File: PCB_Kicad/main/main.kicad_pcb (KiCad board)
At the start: 2 copper layers, 111.8 x 65.4 mm, 52 parts, among them Q1 Q_NMOS_GDS, U1 TL084, U2 TL084, U3 NA555D, U4 FAN7371

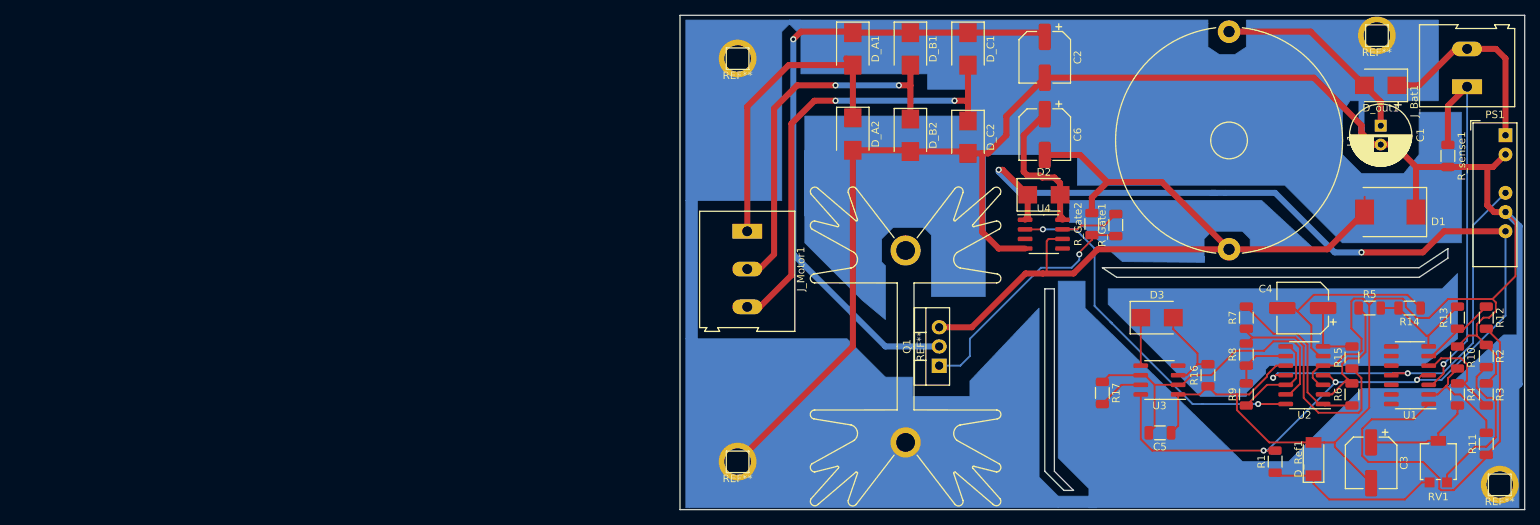
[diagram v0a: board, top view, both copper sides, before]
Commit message: ic tested
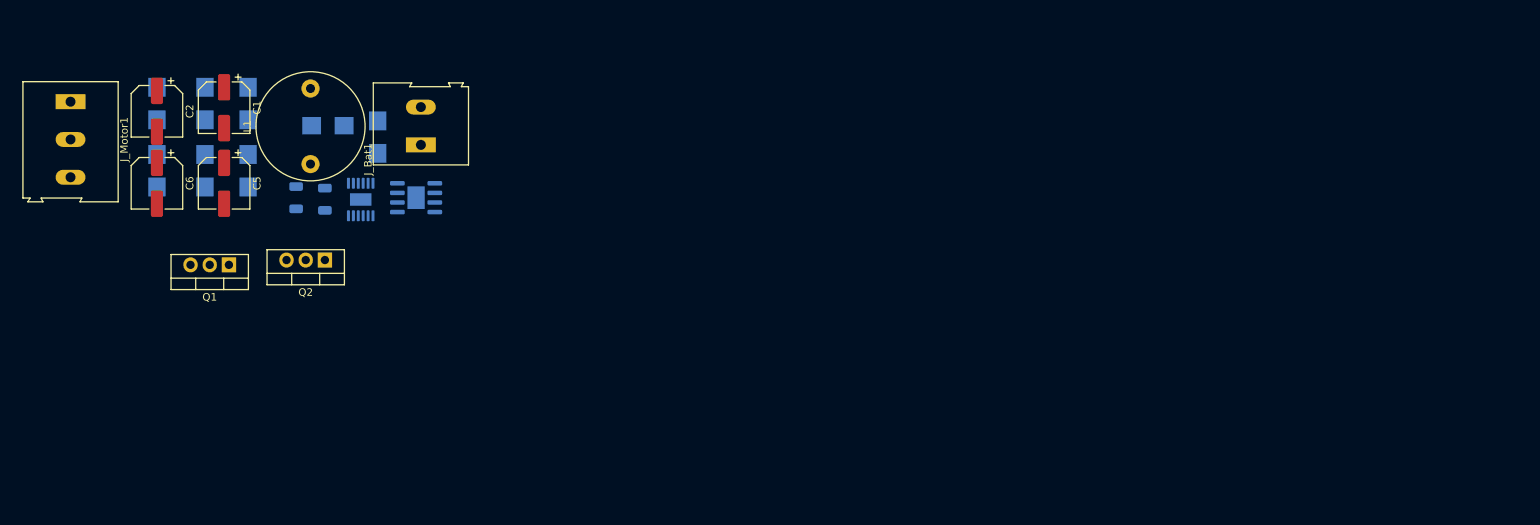
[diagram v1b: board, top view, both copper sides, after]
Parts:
- removed D1: DIODE, Diode_SMD:D_SMC
- removed D2, D3: DIODE, Diode_SMD:D_SMB
- removed D_Ref1: D_Zener_Small, Diode_SMD:D_SOD-128
- removed PS1: IA2412S, Converter_DCDC:Converter_DCDC_XP_POWER-IAxxxxS_THT
- removed R1, R10, R11, R12, R13, R14, R15, R16, R17, R2, R3, R4, R5, R6, R7, R8, R9, R_Gate1, R_Gate2, R_sense1: R_Small_US, Resistor_SMD:R_1206_3216Metric
- removed REF** (x4): Pin_D1.4mm_L8.5mm_W2.8mm_FlatFork, Connector_Pin:Pin_D1.4mm_L8.5mm_W2.8mm_FlatFork
- removed REF**: Heatsink_Fischer_SK129-STS_42x25mm_2xDrill2.5mm, Heatsink:Heatsink_Fischer_SK129-STS_42x25mm_2xDrill2.5mm
- removed RV1: R_POT_TRIM_US, Potentiometer_SMD:Potentiometer_Bourns_3314G_Vertical
- removed U3: NA555D, Package_SO:SOIC-8_3.9x4.9mm_P1.27mm
- removed U4: FAN7371, Package_SO:SOIC-8_3.9x4.9mm_P1.27mm
- added D_Boost1: D_Small, Diode_SMD:D_SMB, B.Cu at (60.3, 28.2)
- added Q2: Q_NMOS_GDS, Package_TO_SOT_THT:TO-220-3_Vertical, F.Cu at (53.3, 44.5)
- C1: value 1mF -> 680uF; footprint Capacitor_THT:CP_Radial_D8.0mm_P2.50mm -> Capacitor_SMD:CP_Elec_6.3x7.7
- C2: value 100uF -> 68uF
- C3: value C_Small -> 2.2nF; footprint Capacitor_SMD:CP_Elec_6.3x7.7 -> Capacitor_SMD:C_1206_3216Metric; moved to B.Cu
- C4: value C_Small -> 2nF; footprint Capacitor_SMD:CP_Elec_6.3x7.7 -> Capacitor_SMD:C_1206_3216Metric; moved to B.Cu
- C5: value C_Small -> 1uF; footprint Capacitor_SMD:C_1206_3216Metric -> Capacitor_SMD:CP_Elec_6.3x7.7
- C6: value C_Small -> 68uF
- D_A1, D_A2, D_B1, D_B2, D_C1, D_C2, D_out1: moved to B.Cu
- L1: value L -> 100uH; footprint Inductor_THT:L_Radial_D29.8mm_P28.80mm_muRATA_1400series -> Inductor_THT:L_Radial_D14.2mm_P10.00mm_Neosid_SD14
- U1: value TL084 -> LTC3854EMSEPBF; footprint Package_SO:SOIC-14_3.9x8.7mm_P1.27mm -> Package_SO:MSOP-12-1EP_3x4mm_P0.65mm_EP1.65x2.85mm; moved to B.Cu
- U2: value TL084 -> ACS70331EESATR-005U3; footprint Package_SO:SOIC-14_3.9x8.7mm_P1.27mm -> Package_SO:SOIC-8-1EP_3.9x4.9mm_P1.27mm_EP2.29x3mm; moved to B.Cu
- moved C1 153.1 mm to (40.0, 24.3)
- moved C3 142.8 mm to (53.3, 36.4), turned to 90 degrees
- moved U1 140.8 mm to (58.1, 36.4), turned to 90 degrees
- moved D_out1 139.4 mm to (53.7, 26.7)
- moved J_Bat1 138.6 mm to (66.0, 29.2)
- moved C4 134.0 mm to (49.5, 36.2), turned to 90 degrees
- moved C5 128.2 mm to (40.0, 34.3), turned to 270 degrees
- moved L1 122.8 mm to (51.4, 31.8), turned to 90 degrees
- moved U2 119.9 mm to (65.4, 36.2)
- moved C2 117.7 mm to (31.1, 24.8)
- moved C6 117.7 mm to (31.1, 34.3)
- moved D_C1 95.5 mm to (43.2, 23.7)
- moved D_C2 95.4 mm to (43.2, 32.6)
- moved Q1 94.9 mm to (40.6, 45.1), turned to 180 degrees
- moved D_B1 93.6 mm to (37.5, 23.7)
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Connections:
- C4 pad 2: Net-(C4-Pad2) -> GND
- C5 pad 1: GND -> SW
- C5 pad 2: PWM_REF -> Net-(C5-Pad2)
- C6 pad 1: Net-(C6-Pad1) -> Net-(C2-Pad1)
- C6 pad 2: Net-(C6-Pad2) -> GND
- L1 pad 2: Net-(C6-Pad2) -> SW
- Q1 pad 1: Net-(Q1-Pad1) -> TG
- Q1 pad 3: Net-(C6-Pad2) -> SW
- U1 pad 1: Net-(R11-Pad1) -> FeedBack
- U1 pad 10: (no net) -> V_Bat
- U1 pad 11: -12V -> GND
- U1 pad 12: (no net) -> GND
- U1 pad 2: Net-(R10-Pad2) -> Net-(C3-Pad1)
- U1 pad 3: V_sense -> Net-(C4-Pad1)
- U1 pad 4: +12V -> Net-(C5-Pad2)
- U1 pad 5: Net-(R3-Pad2) -> TG
- U1 pad 6: Net-(R12-Pad1) -> SW
- U1 pad 7: Net-(R13-Pad2) -> GND
- U1 pad 8: (no net) -> BG
- U1 pad 9: (no net) -> +5V
- U2 pad 1: Net-(R6-Pad1) -> V_sense
- U2 pad 2: Net-(R5-Pad1) -> V_sense
- U2 pad 4: +12V -> GND
- U2 pad 6: Net-(C4-Pad2) -> (no net)
- U2 pad 7: Net-(C4-Pad1) -> (no net)
- U2 pad 8: Net-(R9-Pad1) -> (no net)
- U2 pad 9: Net-(R8-Pad1) -> (no net)
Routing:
- net GND: track 429.3 -> 0.00 mm
- net +12V: track 160.8 -> 0.00 mm, vias 5 -> 0
- net Net-(C6-Pad2): track 106.6 -> 0.00 mm
- net Net-(C2-Pad1): track 87.8 -> 0.00 mm, vias 1 -> 0
- net Net-(D_C1-Pad2): track 59.7 -> 0.00 mm, vias 2 -> 0
- net -12V: track 54.1 -> 0.00 mm, vias 2 -> 0
- net Net-(R11-Pad1): track 53.2 -> 0.00 mm
- net V_sense: track 50.6 -> 0.00 mm, vias 1 -> 0
- net Net-(D_B1-Pad2): track 50.1 -> 0.00 mm, vias 2 -> 0
- net PWM_Gen: track 48.9 -> 0.00 mm, vias 2 -> 0
- net PWM_REF: track 43.7 -> 0.00 mm
- net Net-(D_A1-Pad2): track 41.0 -> 0.00 mm
- net Net-(Q1-Pad1): track 32.9 -> 0.00 mm, vias 1 -> 0
- net Net-(R15-Pad1): track 31.4 -> 0.00 mm
- net Net-(C4-Pad2): track 27.7 -> 0.00 mm
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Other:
- board outline removed
- net class Default: clearance 0.25 -> 0.2; trace_width 0.25 -> 0.2
- rule pad_to_mask_clearance: 0.15 -> 0.12
- rule solder_mask_min_width: 0.15 -> 0.12
- rule trace_clearance: 0.25 -> 0.2

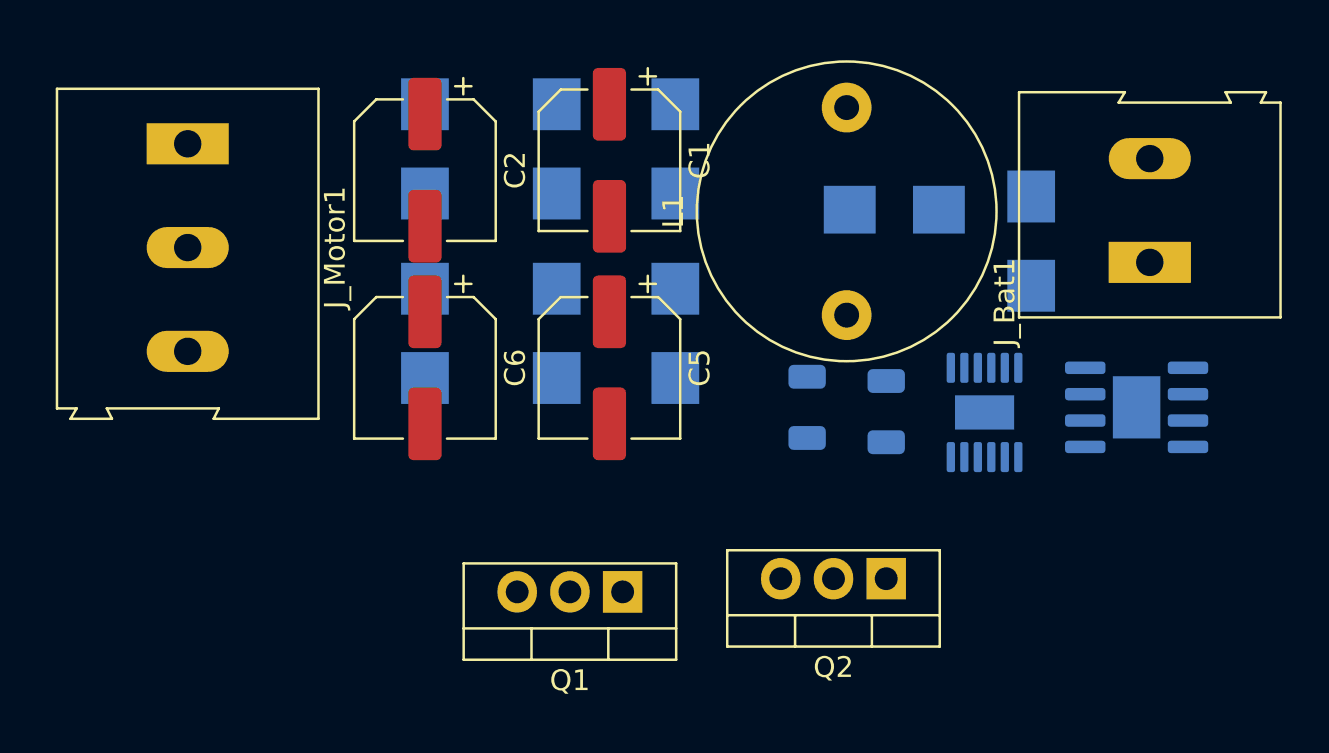
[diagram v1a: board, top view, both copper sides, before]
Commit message: kicad update
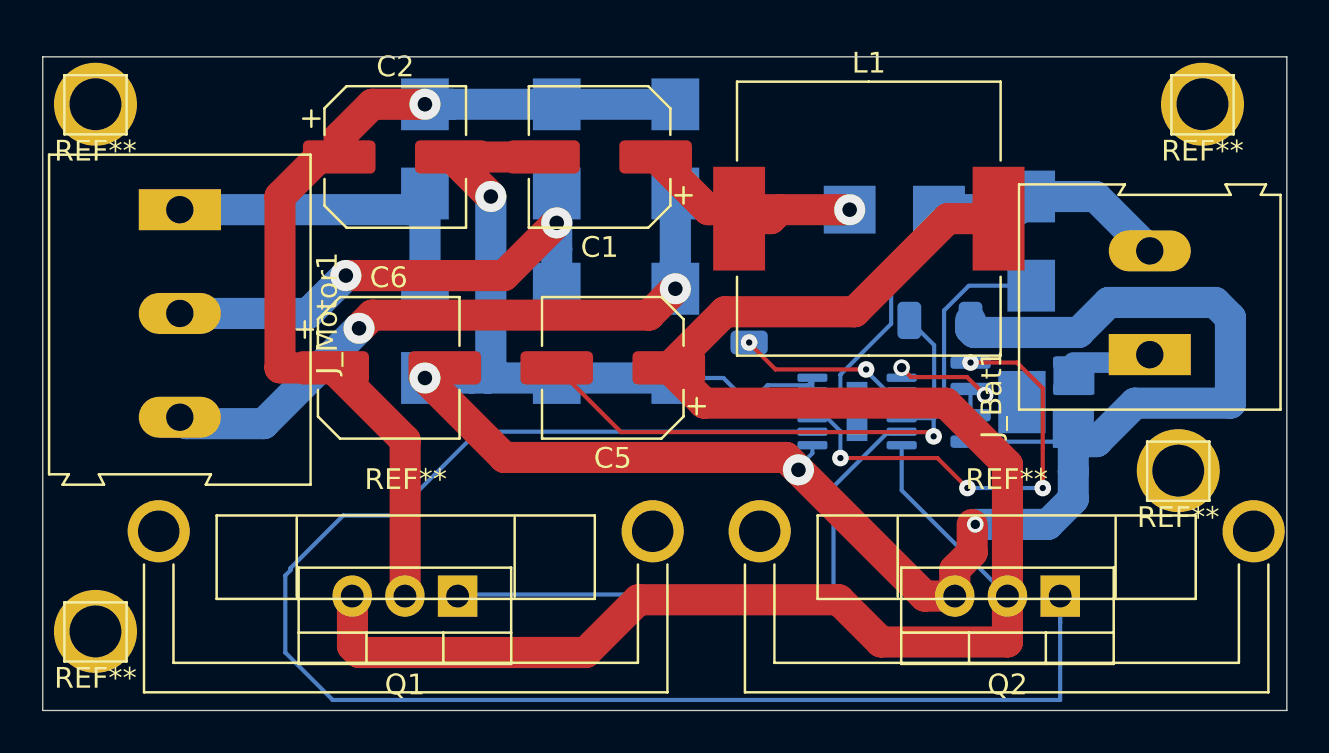
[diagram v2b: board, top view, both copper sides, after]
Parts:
- added REF**: Pin_D1.4mm_L8.5mm_W2.8mm_FlatFork, Connector_Pin:Pin_D1.4mm_L8.5mm_W2.8mm_FlatFork, F.Cu at (67.4, 39.2)
- added REF**: Pin_D1.4mm_L8.5mm_W2.8mm_FlatFork, Connector_Pin:Pin_D1.4mm_L8.5mm_W2.8mm_FlatFork, F.Cu at (68.6, 21.6)
- added REF**: Pin_D1.4mm_L8.5mm_W2.8mm_FlatFork, Connector_Pin:Pin_D1.4mm_L8.5mm_W2.8mm_FlatFork, F.Cu at (15.2, 47.0)
- added REF**: Pin_D1.4mm_L8.5mm_W2.8mm_FlatFork, Connector_Pin:Pin_D1.4mm_L8.5mm_W2.8mm_FlatFork, F.Cu at (15.2, 21.6)
- added REF**: Heatsink_Fischer_FK224xx2201_25x8.3mm, Heatsink:Heatsink_Fischer_FK224xx2201_25x8.3mm, F.Cu at (47.2, 42.2)
- added REF**: Heatsink_Fischer_FK224xx2201_25x8.3mm, Heatsink:Heatsink_Fischer_FK224xx2201_25x8.3mm, F.Cu at (18.3, 42.2)
- L1: footprint Inductor_THT:L_Radial_D14.2mm_P10.00mm_Neosid_SD14 -> Inductor_SMD:L_Wuerth_HCM-1390
- moved Q2 8.42 mm to (61.7, 45.3)
- moved Q1 7.95 mm to (32.7, 45.3)
- moved C4 7.65 mm to (55.9, 32.0), turned to 0 degrees
- moved C3 6.86 mm to (46.7, 34.5), turned to 270 degrees
- moved U1 6.15 mm to (51.9, 36.4), turned to 180 degrees
- moved U2 5.53 mm to (59.9, 35.9)
- moved L1 4.77 mm to (52.5, 27.1), turned to 0 degrees
- moved J_Bat1 4.45 mm to (66.0, 33.7)
- moved J_Motor1 3.20 mm to (19.3, 26.7)
- moved C6 1.74 mm to (29.4, 34.3), turned to 0 degrees
- moved C2 1.56 mm to (29.7, 24.1), turned to 0 degrees
- moved C1 0.50 mm to (39.5, 24.1), turned to 180 degrees
- moved C5 0.16 mm to (40.2, 34.3), turned to 180 degrees
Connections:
- Q2 pad 1: Bg -> Net-(Q2-Pad1)
- U1 pad 8: BG -> Net-(Q2-Pad1)
- U1 pad 9: +5V -> Net-(U1-Pad9)
- U2 pad 7: (no net) -> FeedBack
- U2 pad 8: (no net) -> Net-(U1-Pad9)
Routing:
- net GND: track 0.00 -> 113.3 mm, vias 0 -> 4
- net SW: track 0.00 -> 91.1 mm
- net Net-(Q2-Pad1): track 0.00 -> 76.8 mm
- net Net-(C2-Pad1): track 0.00 -> 44.6 mm, vias 0 -> 1
- net Net-(C5-Pad2): track 0.00 -> 32.1 mm, vias 0 -> 1
- net Net-(D_C1-Pad2): track 0.00 -> 31.3 mm, vias 0 -> 2
- net TG: track 0.00 -> 27.7 mm
- net Net-(D_B1-Pad2): track 0.00 -> 24.6 mm, vias 0 -> 2
- net V_Bat: track 0.00 -> 23.9 mm
- net Net-(U1-Pad9): track 0.00 -> 22.6 mm, vias 0 -> 4
- net Net-(D_A1-Pad2): track 0.00 -> 16.7 mm
- net Net-(C1-Pad1): track 0.00 -> 12.5 mm, vias 0 -> 1
- net Net-(C3-Pad1): track 0.00 -> 8.48 mm, vias 0 -> 2
- net Net-(C4-Pad1): track 0.00 -> 6.07 mm
- net V_sense: track 0.00 -> 5.11 mm
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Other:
- board outline added: 59.9 x 31.5 mm

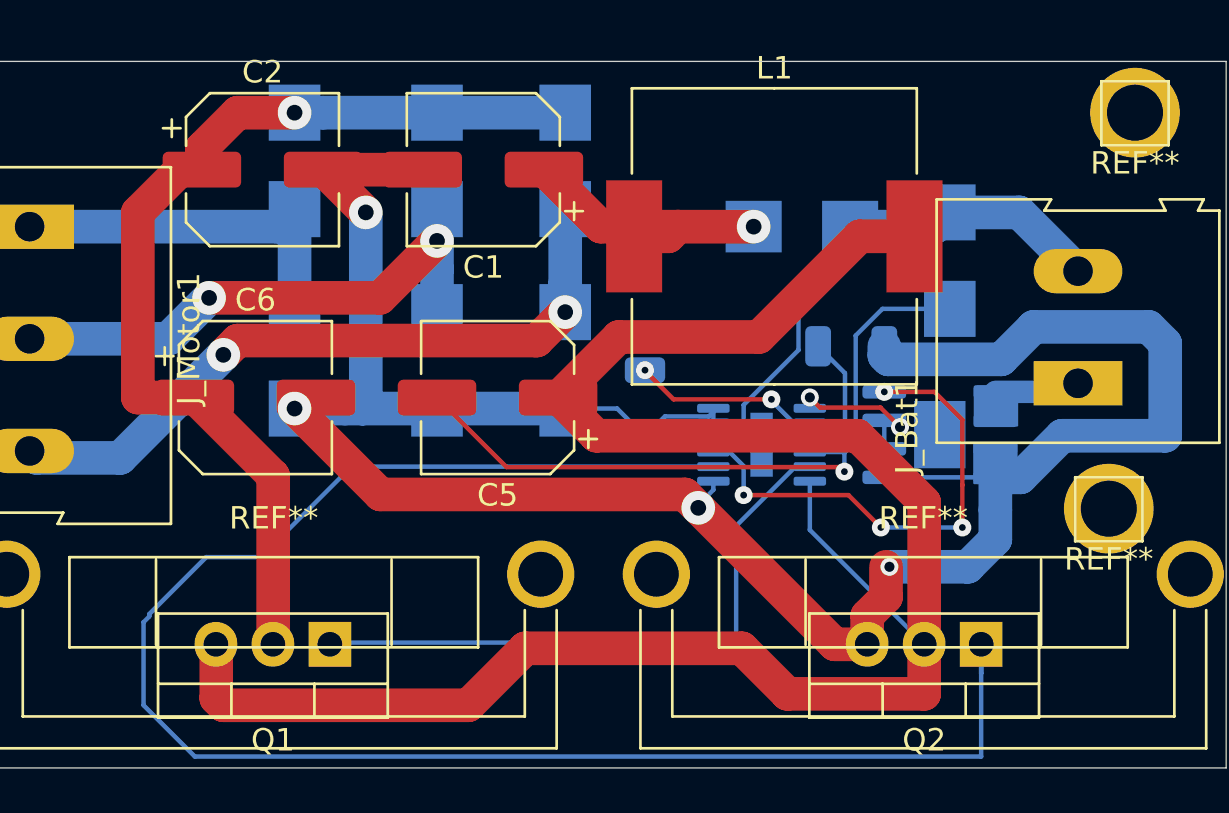
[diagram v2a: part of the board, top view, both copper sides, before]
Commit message: model update
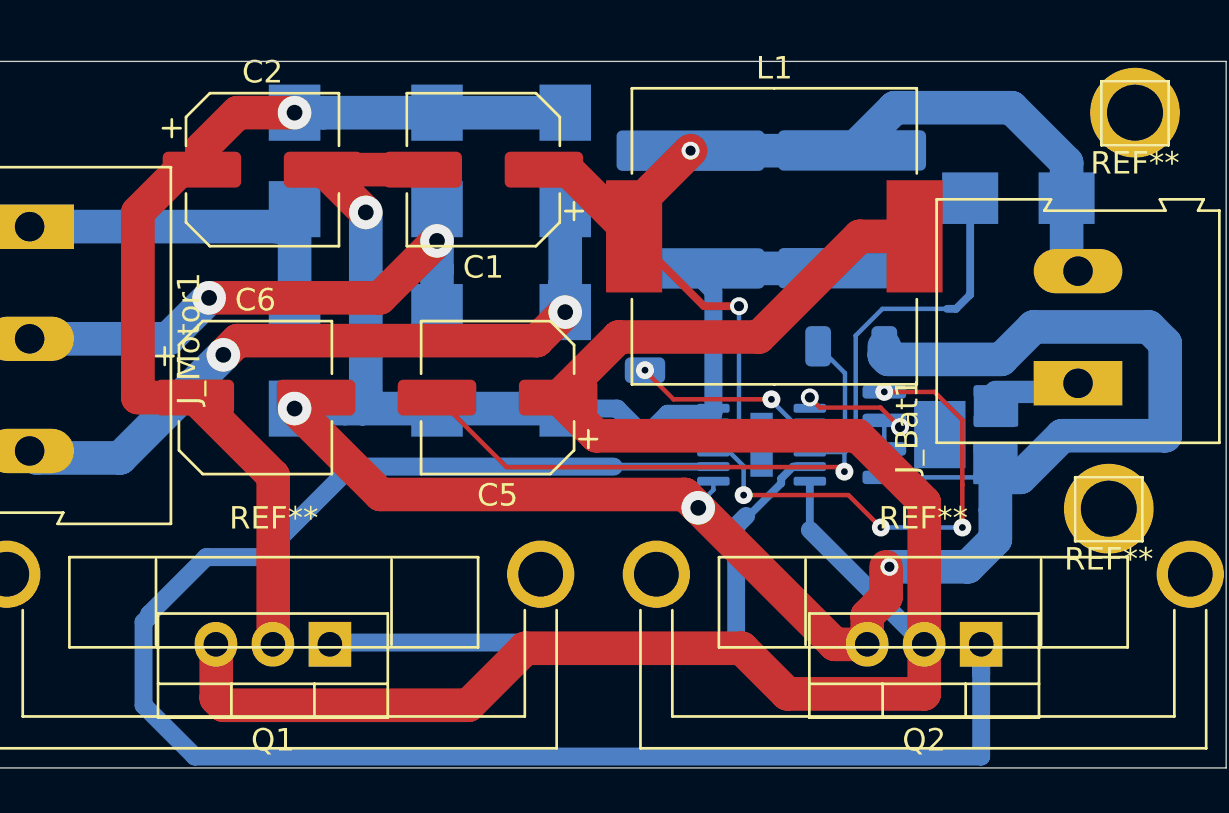
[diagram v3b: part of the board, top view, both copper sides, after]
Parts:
- removed D_out1: D_Schottky, Diode_SMD:D_SMB
- added C7: 4.7uF, Capacitor_SMD:C_2225_5664Metric_Pad1.80x6.60mm_HandSolder, B.Cu at (48.8, 25.9)
- added C8: 4.7uF, Capacitor_SMD:C_2225_5664Metric_Pad1.80x6.60mm_HandSolder, B.Cu at (56.0, 25.9)
- moved D_Boost1 4.14 mm to (63.4, 25.4), turned to 0 degrees
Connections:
- C1 pad 1: Net-(C1-Pad1) -> V_Bat
- L1 pad 1: Net-(C1-Pad1) -> V_Bat
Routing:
- net V_Bat: track 23.9 -> 46.4 mm, vias 0 -> 2
- net GND: track 113.3 -> 130.8 mm
- net Net-(C1-Pad1): track 12.5 -> 0.00 mm, vias 1 -> 0
- net Net-(C5-Pad2): track 32.1 -> 37.7 mm
